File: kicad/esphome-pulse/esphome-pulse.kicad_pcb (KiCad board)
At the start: 2 copper layers, 33 x 24.6 mm, 3 parts, among them J2 AudioJack2_Ground

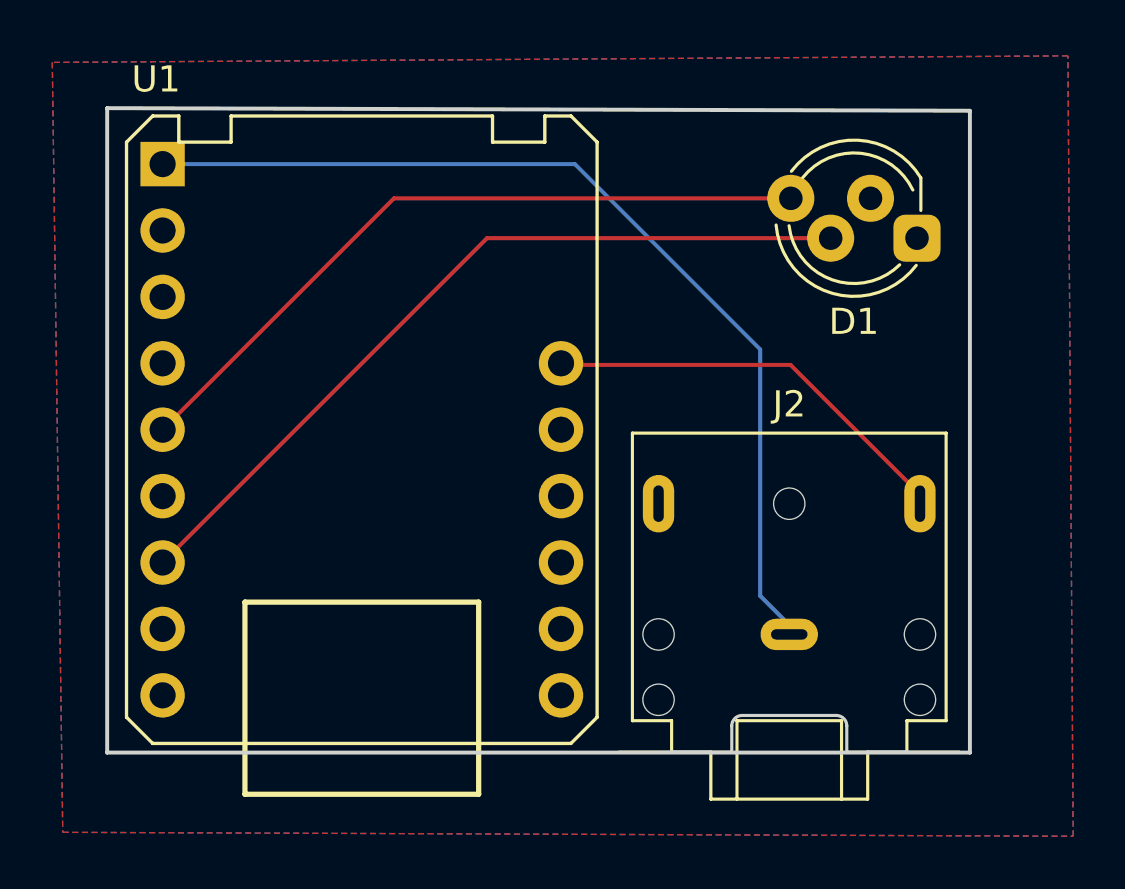
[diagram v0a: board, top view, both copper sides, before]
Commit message: Sent to production
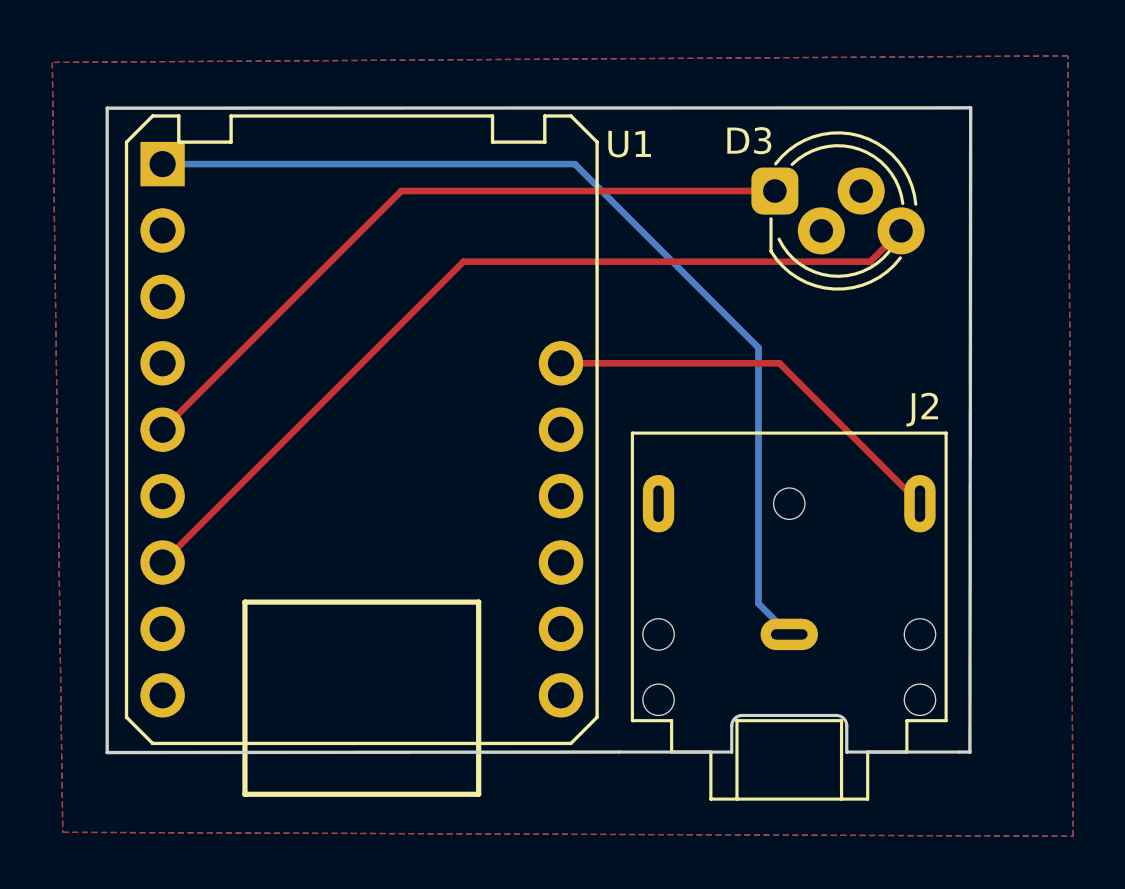
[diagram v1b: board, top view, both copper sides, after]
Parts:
- removed D1: APA-106-F5, LED_THT:LED_D5.0mm-4_RGB_Staggered_Pins
- added D3: WS2812B_THT, LED_THT:LED_D5.0mm-4_RGB_Staggered_Pins, F.Cu at (94.5, 71.8)
- J2: value AudioJack2_Ground -> AudioJack2
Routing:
- net +5V: track 30.9 -> 33.8 mm
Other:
- board size 33 x 24.6 mm -> 33 x 24.7 mm
- board text added: "ESPHome Pulse"
- board text added: "openenergy.com.au esphome-pulse April 2025 v1.0"
